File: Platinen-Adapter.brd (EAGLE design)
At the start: 26 x 100 mm, 2 parts, among them X1 MAC64L

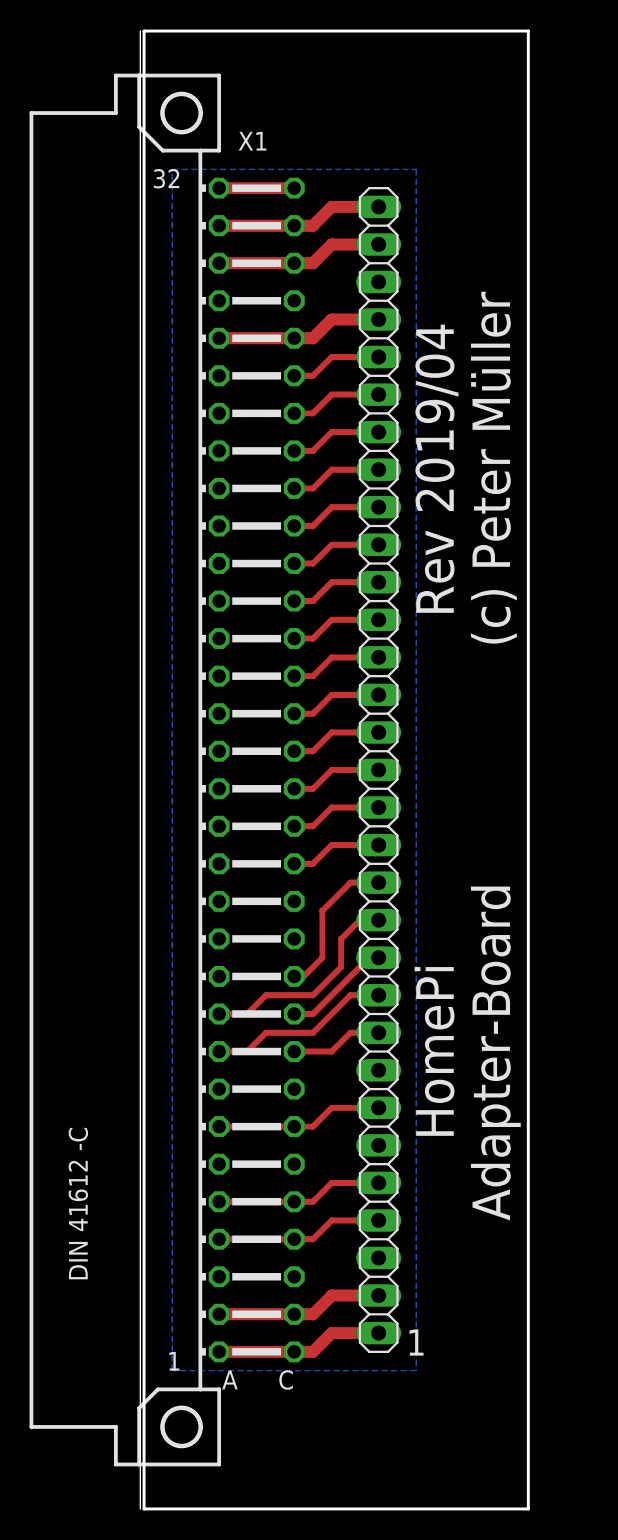
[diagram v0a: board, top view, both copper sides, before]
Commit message: Layouts angepasst
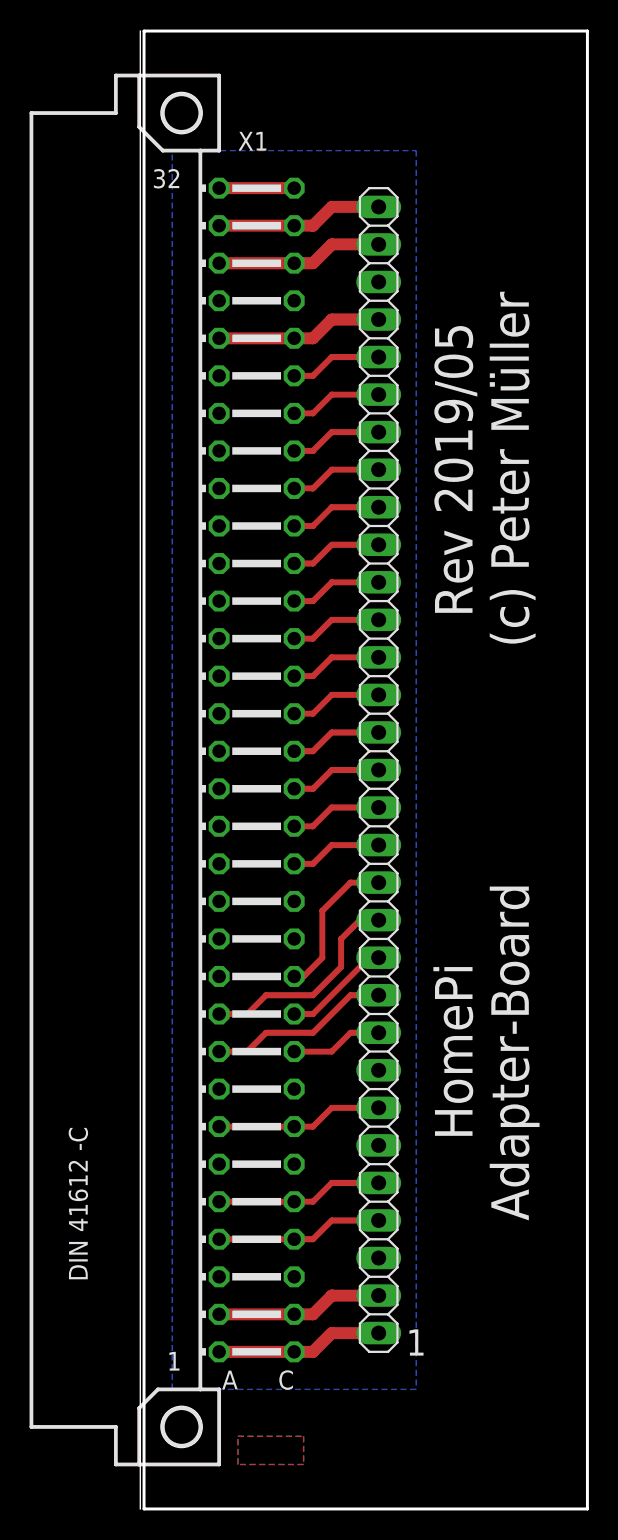
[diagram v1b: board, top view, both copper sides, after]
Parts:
- added U$2: (no value), cryCode-Logo:30MM
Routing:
- added copper zone on layer 16, net BOT
- added copper zone on layer 1, net TOP
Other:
- board size 26 x 100 mm -> 30 x 100 mm
- board text added: "BOT"
- board text added: "Rev 2019/05 (c) Peter Müller"
- board text added: "TOP"
- board text removed: "Rev 2019/04 (c) Peter Müller"
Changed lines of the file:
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@@
 <layer number="51" name="tDocu" color="7" fill="1" visible="yes" active="yes"/>
 <layer number="52" name="bDocu" color="7" fill="1" visible="yes" active="yes"/>
+<layer number="53" name="tGND_GNDA" color="7" fill="1" visible="no" active="no"/>
+<layer number="54" name="bGND_GNDA" color="7" fill="1" visible="no" active="no"/>
+<layer number="56" name="wert" color="7" fill="1" visible="no" active="no"/>
 <layer number="90" name="Modules" color="5" fill="1" visible="no" active="no"/>
 <layer number="91" name="Nets" color="2" fill="1" visible="no" active="no"/>
@@
 <layer number="98" name="Guide" color="6" fill="1" visible="no" active="no"/>
 <layer number="99" name="SpiceOrder" color="5" fill="1" visible="no" active="no"/>
+<layer number="100" name="Muster" color="7" fill="1" visible="yes" active="yes"/>
+<layer number="101" name="Flex-Kleb" color="7" fill="1" visible="yes" active="yes"/>
+<layer number="102" name="fp2" color="7" fill="1" visible="yes" active="yes"/>
+<layer number="103" name="fp3" color="7" fill="1" visible="yes" active="yes"/>
+<layer number="104" name="fp4" color="7" fill="1" visible="yes" active="yes"/>
+<layer number="105" name="Beschreib" color="7" fill="1" visible="yes" active="yes"/>
+<layer number="106" name="BGA-Top" color="7" fill="1" visible="yes" active="yes"/>
+<layer number="107" name="BD-Top" color="7" fill="1" visible="yes" active="yes"/>
+<layer number="108" name="fp8" color="7" fill="1" visible="yes" active="yes"/>
+<layer number="109" name="fp9" color="7" fill="1" visible="yes" active="yes"/>
+<layer number="110" name="fp0" color="7" fill="1" visible="yes" active="yes"/>
+<layer number="111" name="bdokum" color="7" fill="1" visible="yes" active="yes"/>
+<layer number="116" name="Patch_BOT" color="7" fill="1" visible="yes" active="yes"/>
+<layer number="121" name="tTestdril" color="7" fill="1" visible="yes" active="yes"/>
+<layer number="122" name="bTestdril" color="7" fill="1" visible="yes" active="yes"/>
+<layer number="123" name="tTestmark" color="7" fill="1" visible="yes" active="yes"/>
+<layer number="124" name="bTestmark" color="7" fill="1" visible="yes" active="yes"/>
+<layer number="125" name="tNamesSMD" color="7" fill="1" visible="yes" active="yes"/>
+<layer number="126" name="bNamesSMD" color="7" fill="1" visible="yes" active="yes"/>
+<layer number="127" name="tValueSMD" color="7" fill="1" visible="yes" active="yes"/>
+<layer number="128" name="bValueSMD" color="7" fill="1" visible="yes" active="yes"/>
+<layer number="131" name="tAdjust" color="7" fill="1" visible="yes" active="yes"/>
+<layer number="132" name="bAdjust" color="7" fill="1" visible="yes" active="yes"/>
+<layer number="144" name="Drill_legend" color="7" fill="1" visible="no" active="yes"/>
+<layer number="151" name="tDocuSMD" color="7" fill="1" visible="yes" active="yes"/>
+<layer number="152" name="bDocuSMD" color="7" fill="1" visible="yes" active="yes"/>
+<layer number="199" name="Contour" color="7" fill="1" visible="yes" active="yes"/>
+<layer number="200" name="200bmp" color="1" fill="10" visible="yes" active="yes"/>
+<layer number="201" name="201bmp" color="7" fill="1" visible="yes" active="yes"/>
+<layer number="202" name="202bmp" color="7" fill="1" visible="yes" active="yes"/>
+<layer number="203" name="203bmp" color="7" fill="1" visible="yes" active="yes"/>
+<layer number="204" name="204bmp" color="7" fill="1" visible="yes" active="yes"/>
+<layer number="205" name="205bmp" color="7" fill="1" visible="yes" active="yes"/>
+<layer number="206" name="206bmp" color="7" fill="1" visible="yes" active="yes"/>
+<layer number="207" name="207bmp" color="7" fill="1" visible="yes" active="yes"/>
+<layer number="208" name="208bmp" color="7" fill="1" visible="yes" active="yes"/>
+<layer number="209" name="209bmp" color="7" fill="1" visible="yes" active="yes"/>
+<layer number="210" name="210bmp" color="7" fill="1" visible="yes" active="yes"/>
+<layer number="211" name="211bmp" color="7" fill="1" visible="no" active="yes"/>
+<layer number="212" name="212bmp" color="7" fill="1" visible="no" active="yes"/>
+<layer number="213" name="213bmp" color="7" fill="1" visible="no" active="yes"/>
+<layer number="214" name="214bmp" color="7" fill="1" visible="no" active="yes"/>
+<layer number="215" name="215bmp" color="7" fill="1" visible="no" active="yes"/>
+<layer number="216" name="216bmp" color="7" fill="1" visible="no" active="yes"/>
+<layer number="217" name="217bmp" color="18" fill="1" visible="no" active="no"/>
+<layer number="218" name="218bmp" color="19" fill="1" visible="no" active="no"/>
+<layer number="219" name="219bmp" color="20" fill="1" visible="no" active="no"/>
+<layer number="220" name="220bmp" color="21" fill="1" visible="no" active="no"/>
+<layer number="221" name="221bmp" color="22" fill="1" visible="no" active="no"/>
+<layer number="222" name="222bmp" color="23" fill="1" visible="no" active="no"/>
+<layer number="223" name="223bmp" color="24" fill="1" visible="no" active="no"/>
+<layer number="224" name="224bmp" color="25" fill="1" visible="no" active="no"/>
 <layer number="250" name="Descript" color="3" fill="1" visible="no" active="no"/>
 <layer number="251" name="SMDround" color="12" fill="11" visible="no" active="no"/>
+<layer number="254" name="OrgLBR" color="7" fill="1" visible="yes" active="yes"/>
 </layers>
 <board>
 <plain>
-<wire x1="0" y1="-0.47" x2="26" y2="-0.47" width="0.2" layer="20"/>
-<wire x1="26" y1="-0.47" x2="26" y2="99.53" width="0.2" layer="20"/>
-<wire x1="26" y1="99.53" x2="0" y2="99.53" width="0.2" layer="20"/>
+<wire x1="0" y1="-0.47" x2="30" y2="-0.47" width="0.2" layer="20"/>
+<wire x1="30" y1="-0.47" x2="30" y2="99.53" width="0.2" layer="20"/>
+<wire x1="30" y1="99.53" x2="0" y2="99.53" width="0.2" layer="20"/>
 <wire x1="0" y1="99.53" x2="0" y2="-0.47" width="0.2" layer="20"/>
-<dimension x1="15.875" y1="48.26" x2="26" y2="48.26" x3="20.9375" y3="-6.35" textsize="1.778" layer="47"/>
-<dimension x1="0" y1="-0.47" x2="0" y2="99.53" x3="-16.51" y3="49.53" textsize="1.778" layer="47"/>
-<dimension x1="0" y1="-0.47" x2="26" y2="-0.47" x3="13" y3="-12.7" textsize="1.778" layer="47"/>
-<text x="18.415" y="69.85" size="2.54" layer="25" font="vector" ratio="15" rot="R90" align="top-center">Rev 2019/04
+<dimension x1="15.875" y1="48.26" x2="30" y2="48.26" x3="22.9375" y3="-6.35" textsize="1.778" layer="47" visible="yes"/>
+<dimension x1="0" y1="-0.47" x2="0" y2="99.53" x3="-16.51" y3="49.53" textsize="1.778" layer="47" visible="yes"/>
+<dimension x1="0" y1="-0.47" x2="30" y2="-0.47" x3="15" y3="-12.7" textsize="1.778" layer="47" visible="yes"/>
+<text x="19.685" y="69.85" size="2.54" layer="25" font="vector" ratio="15" rot="R90" align="top-center">Rev 2019/05
 (c) Peter Müller</text>
-<text x="18.415" y="30.48" size="2.54" layer="25" font="vector" ratio="15" rot="R90" align="top-center">HomePi
+<text x="19.685" y="30.48" size="2.54" layer="25" font="vector" ratio="15" rot="R90" align="top-center">HomePi
 Adapter-Board</text>
 <text x="18.415" y="10.795" size="1.778" layer="25" font="vector" ratio="10" align="center">1</text>
-<text x="18.415" y="69.85" size="2.54" layer="26" font="vector" ratio="15" rot="SMR270" align="top-center">HomePi
-Adapter-Board</text>
-<text x="18.415" y="30.48" size="2.54" layer="26" font="vector" ratio="15" rot="SMR270" align="top-center">Rev 2019/04
-(c) Peter Müller</text>
+<text x="10.16" y="2.8575" size="1.27" layer="42" font="vector" ratio="15" rot="MR0">BOT</text>
+<text x="10.16" y="2.8575" size="1.27" layer="41" font="vector" ratio="15" align="bottom-right">TOP</text>
 </plain>
 <attributes>
@@
 <attribute name="VALUE" x="-5.08" y="60.9854" size="1.27" layer="27" ratio="10" rot="R270"/>
 </element>
+<element name="U$2" library="cryCode-Logo" package="30MM" value="" x="26.67" y="64.77" rot="MR270"/>
 </elements>
 <signals>
@@
 <signal name="GND">
 <polygon width="0.254" layer="16" isolate="0.254">
-<vertex x="1.905" y="90.17"/>
-<vertex x="18.415" y="90.17"/>
-<vertex x="18.415" y="8.89"/>
-<vertex x="1.905" y="8.89"/>
+<vertex x="1.905" y="91.44"/>
+<vertex x="18.415" y="91.44"/>
+<vertex x="18.415" y="7.62"/>
+<vertex x="1.905" y="7.62"/>
 </polygon>
 <contactref element="SV1" pad="29"/>
@@
 <contactref element="X1" pad="A26"/>
 </signal>
+<signal name="TOP">
+<polygon width="0.254" layer="1" orphans="yes">
+<vertex x="6.35" y="4.445"/>
+<vertex x="10.795" y="4.445"/>
+<vertex x="10.795" y="2.54"/>
+<vertex x="6.35" y="2.54"/>
+</polygon>
+</signal>
+<signal name="BOT">
+<polygon width="0.254" layer="16" orphans="yes">
+<vertex x="6.35" y="4.445"/>
+<vertex x="10.795" y="4.445"/>
+<vertex x="10.795" y="2.54"/>
+<vertex x="6.35" y="2.54"/>
+</polygon>
+</signal>
 </signals>
